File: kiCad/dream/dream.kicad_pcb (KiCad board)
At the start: 2 copper layers, 58.8 x 78 mm, 35 parts, among them IC1 TGS2611-C00, J1 GPIO, J2 Qwiic_Vertical, J3 679305124022, J4 Qwiic_Vertical, J5 M20-7830542, J6 Qwiic_Vertical, J7 5013310607, J8 Qwiic_Vertical, J9 Qwiic_Vertical, Q1 BSS138, U1 AP2112K-3.3, U2 BME280, U3 INA219BxDCN, U4 12401610E4-2A

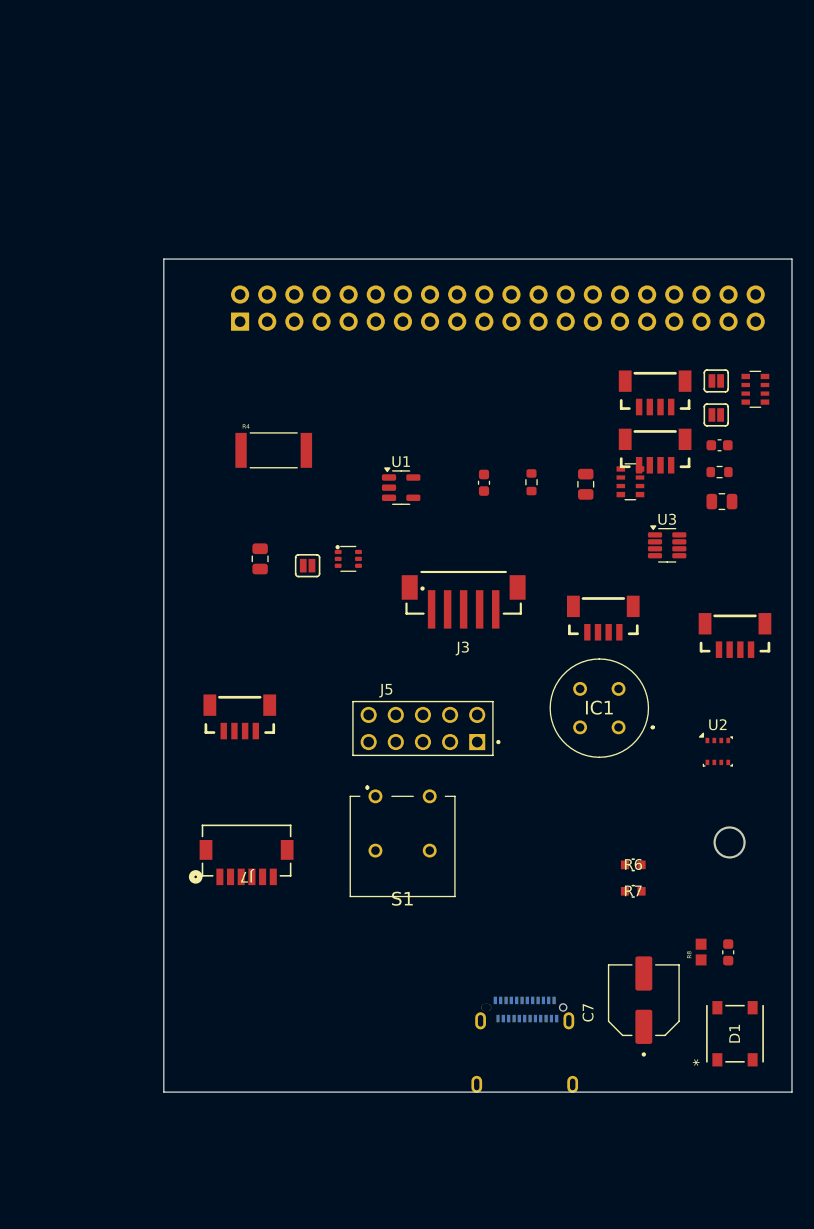
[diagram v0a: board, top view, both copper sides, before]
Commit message: dream updates
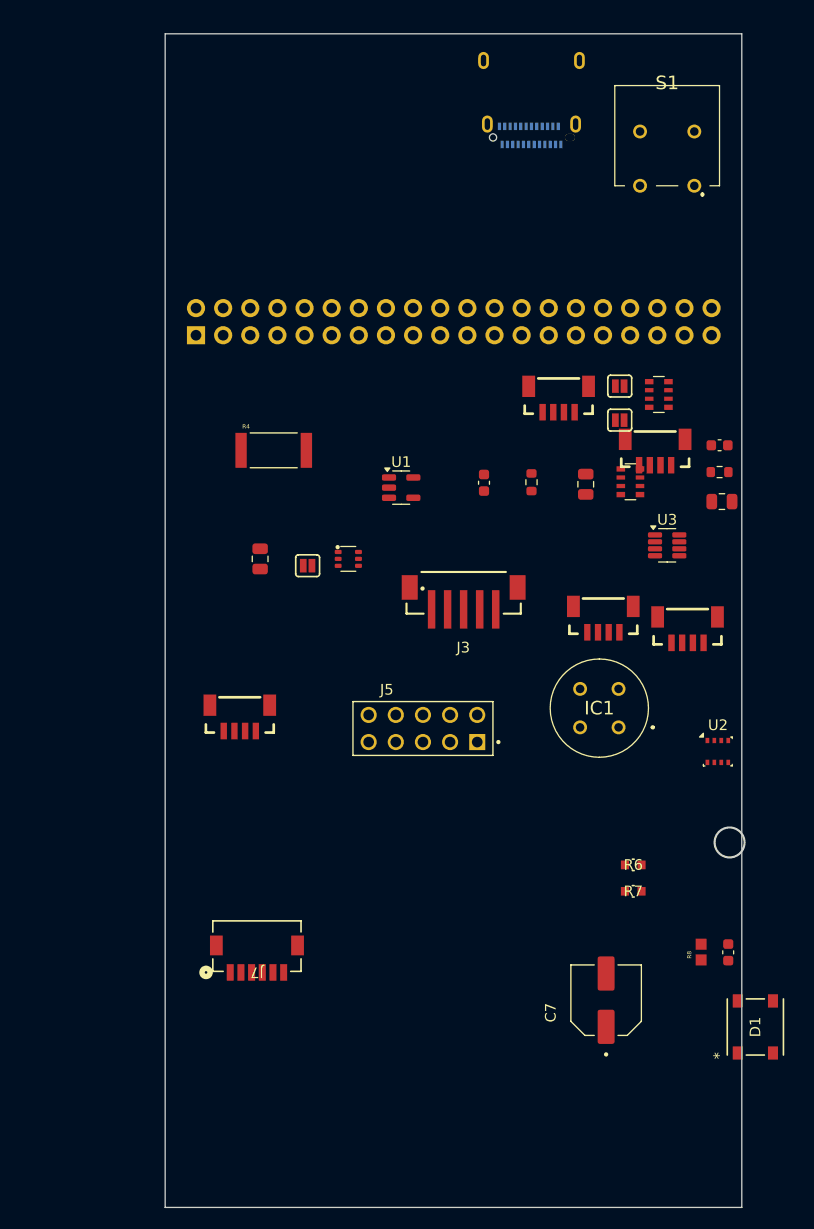
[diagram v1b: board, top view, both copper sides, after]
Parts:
- moved U4 90.2 mm to (134.3, 45.4), turned to 0 degrees
- moved S1 64.5 mm to (149.5, 54.3), turned to 180 degrees
- moved J8 9.05 mm to (136.8, 74.0)
- moved JP2 9.05 mm to (142.5, 73.0)
- moved JP3 9.05 mm to (142.5, 76.2)
- moved R5 9.05 mm to (146.2, 73.8)
- moved J7 9.00 mm to (108.6, 125.5)
- moved J4 4.49 mm to (148.9, 95.6)
- moved J1 4.32 mm to (102.9, 68.3)
- moved C7 3.53 mm to (141.3, 130.5)
- moved D1 2.01 mm to (155.2, 133.0)
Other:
- board size 58.8 x 78 mm -> 54.2 x 109.9 mm

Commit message: major updates
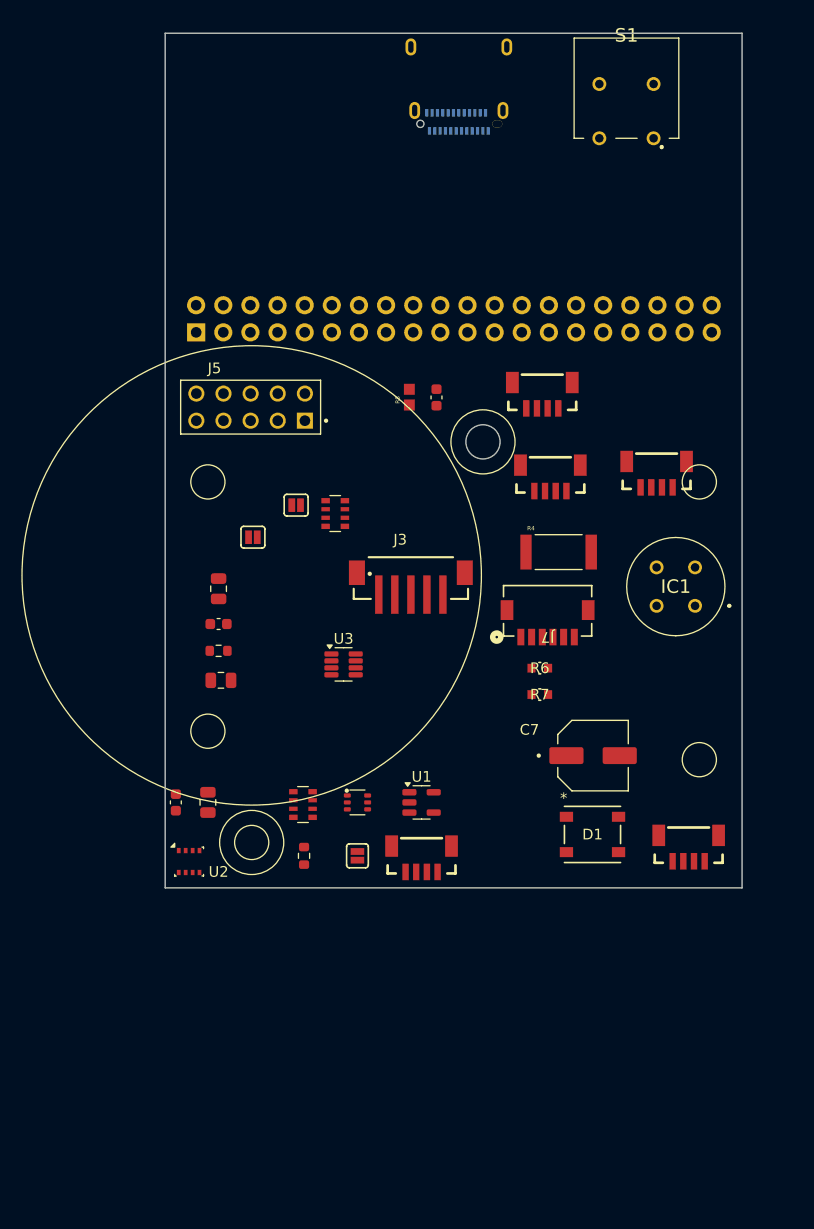
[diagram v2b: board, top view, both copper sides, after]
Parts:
- moved C6 58.7 mm to (125.4, 74.1)
- moved R8 58.7 mm to (122.9, 74.1)
- moved U2 50.5 mm to (102.2, 117.5)
- moved C5 49.8 mm to (105.0, 95.3)
- moved R3 49.8 mm to (105.0, 97.8)
- moved C4 49.8 mm to (105.2, 100.6)
- moved R1 43.0 mm to (112.9, 112.2)
- moved C1 41.6 mm to (101.0, 112.0)
- moved J7 41.5 mm to (135.8, 94.1)
- moved J2 41.4 mm to (135.3, 73.6)
- moved R2 40.9 mm to (113.0, 117.0)
- moved J9 37.2 mm to (149.0, 116.0)
- moved JP3 36.0 mm to (108.2, 87.2)
- moved C2 35.7 mm to (105.0, 92.0)
- moved J5 34.1 mm to (108.0, 75.0)
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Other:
- board size 54.2 x 109.9 mm -> 54 x 80 mm
